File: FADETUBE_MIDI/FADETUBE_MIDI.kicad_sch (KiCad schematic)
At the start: 7 parts, among them J1 B8B-XH-A, J2 B8B-XH-A, J3 B8B-PH-K-S, J4 B8B-PH-K-S, U1 Sparkfun_Pro_Micro

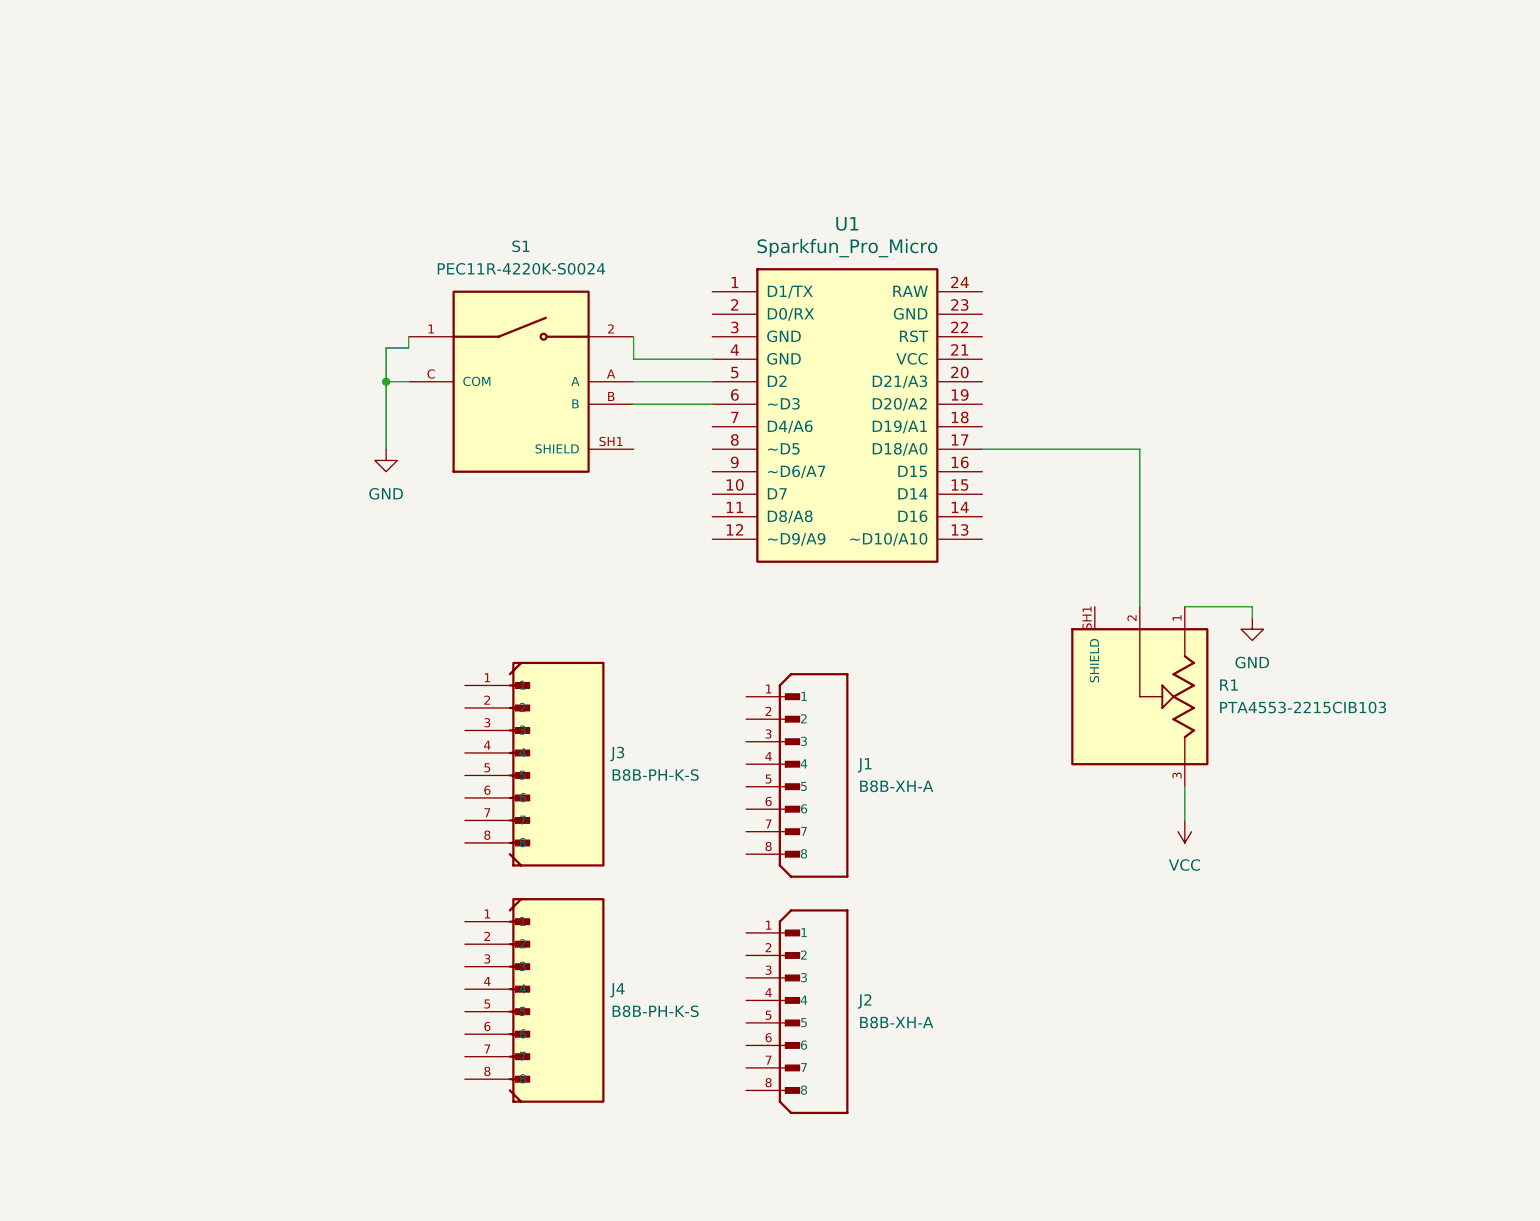
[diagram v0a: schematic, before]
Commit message: updates
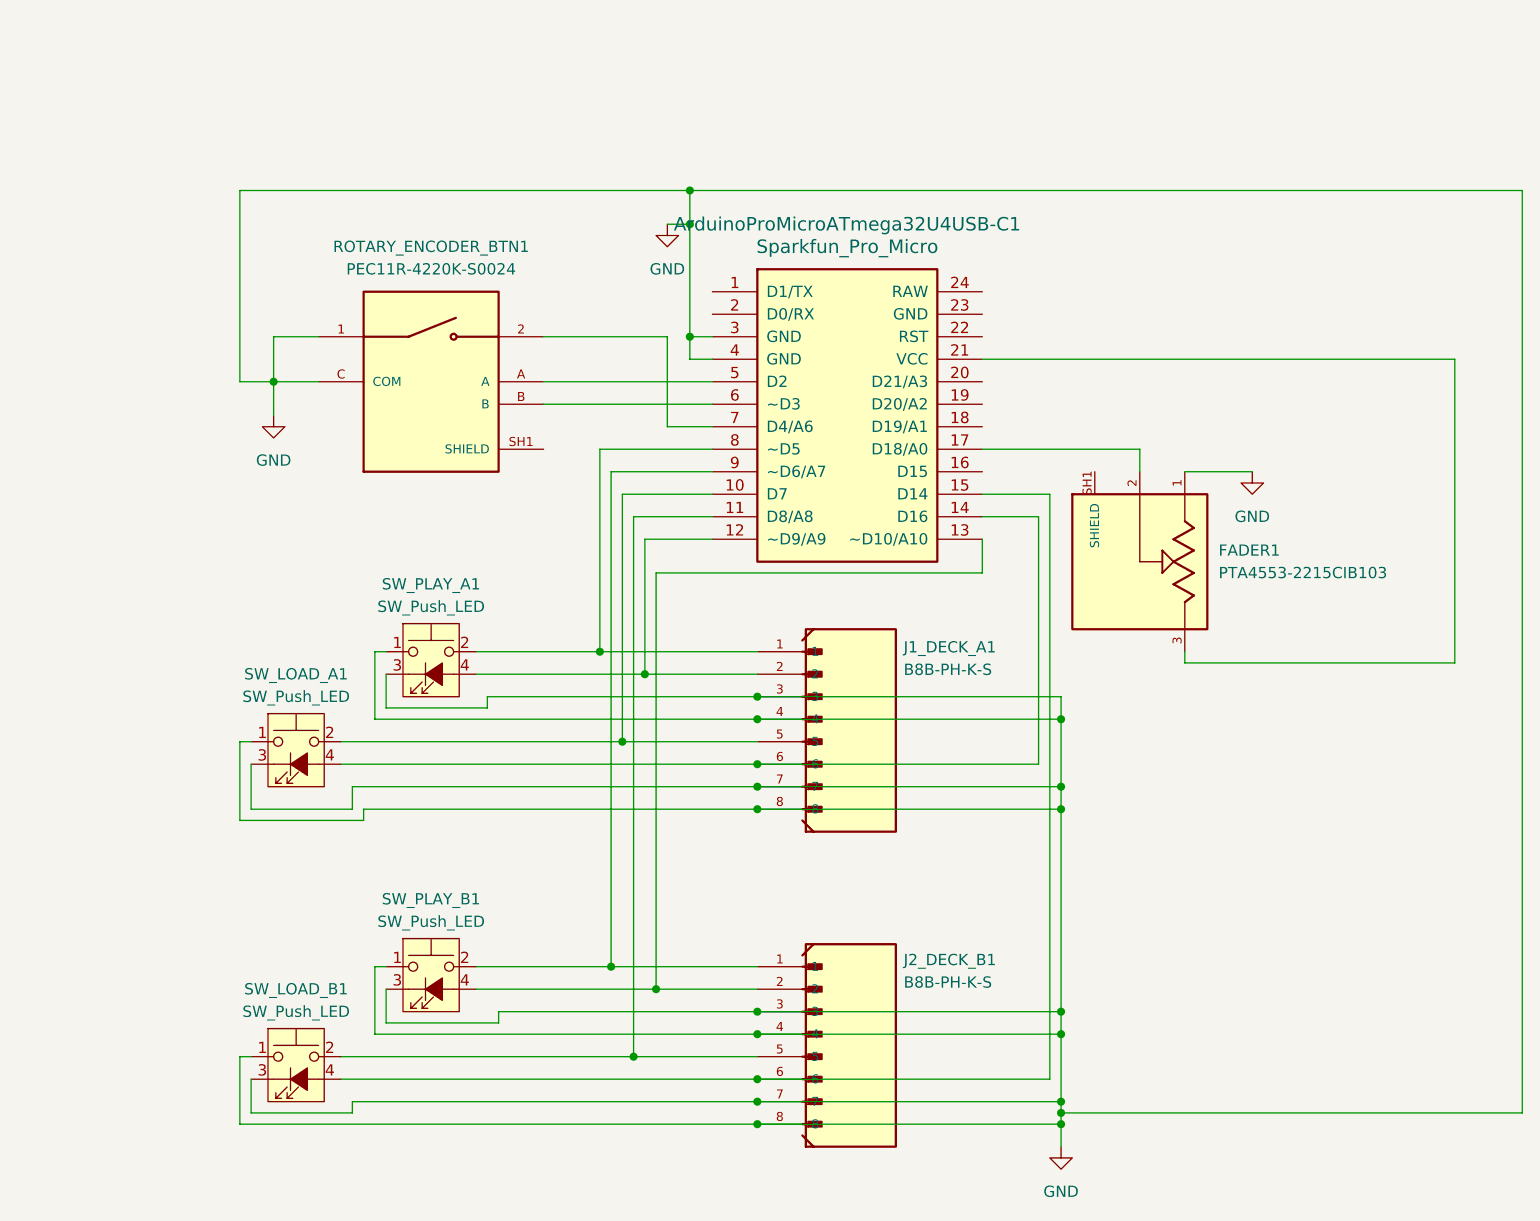
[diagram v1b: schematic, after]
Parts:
- removed J1, J2: B8B-XH-A, FADETUBE_LIBRARY:JST_B8B-XH-A, symbol FADETUBE_LIBRARY:B8B-XH-A
- added SW_LOAD_A1, SW_LOAD_B1, SW_PLAY_A1, SW_PLAY_B1: SW_Push_LED, symbol Switch:SW_Push_LED
- renumbered U1 to ArduinoProMicroATmega32U4USB-C1, R1 to FADER1, J3 to J1_DECK_A1, J4 to J2_DECK_B1, S1 to ROTARY_ENCODER_BTN1
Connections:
- net VCC is gone; now on an unnamed net: FADER1.3
- net GND: now also ArduinoProMicroATmega32U4USB-C1.3 (GND), ArduinoProMicroATmega32U4USB-C1.4 (GND), J1_DECK_A1.3, J1_DECK_A1.4, J1_DECK_A1.7, J1_DECK_A1.8, J2_DECK_B1.3, J2_DECK_B1.4, J2_DECK_B1.7, J2_DECK_B1.8, SW_LOAD_A1.1, SW_LOAD_A1.3 (K), SW_LOAD_B1.1, SW_LOAD_B1.3 (K), SW_PLAY_A1.1, SW_PLAY_A1.3 (K), SW_PLAY_B1.1, SW_PLAY_B1.3 (K)
- net at J1_DECK_A1.1: now also ArduinoProMicroATmega32U4USB-C1.8 (~D5), SW_PLAY_A1.2
- net at J1_DECK_A1.2: now also ArduinoProMicroATmega32U4USB-C1.12 (~D9/A9), SW_PLAY_A1.4 (A)
- net at J1_DECK_A1.5: now also ArduinoProMicroATmega32U4USB-C1.10 (D7), SW_LOAD_A1.2
- net at J1_DECK_A1.6: now also ArduinoProMicroATmega32U4USB-C1.14 (D16), SW_LOAD_A1.4 (A)
- net at J2_DECK_B1.1: now also ArduinoProMicroATmega32U4USB-C1.9 (~D6/A7), SW_PLAY_B1.2
- net at J2_DECK_B1.2: now also ArduinoProMicroATmega32U4USB-C1.13 (~D10/A10), SW_PLAY_B1.4 (A)
- net at J2_DECK_B1.5: now also ArduinoProMicroATmega32U4USB-C1.11 (D8/A8), SW_LOAD_B1.2
- net at J2_DECK_B1.6: now also ArduinoProMicroATmega32U4USB-C1.15 (D14), SW_LOAD_B1.4 (A)
- net at ROTARY_ENCODER_BTN1.2: now also ArduinoProMicroATmega32U4USB-C1.7 (D4/A6); no longer ArduinoProMicroATmega32U4USB-C1.4 (GND)
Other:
- moved on the sheet: FADER1, J1_DECK_A1, J2_DECK_B1, ROTARY_ENCODER_BTN1

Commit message: test smd
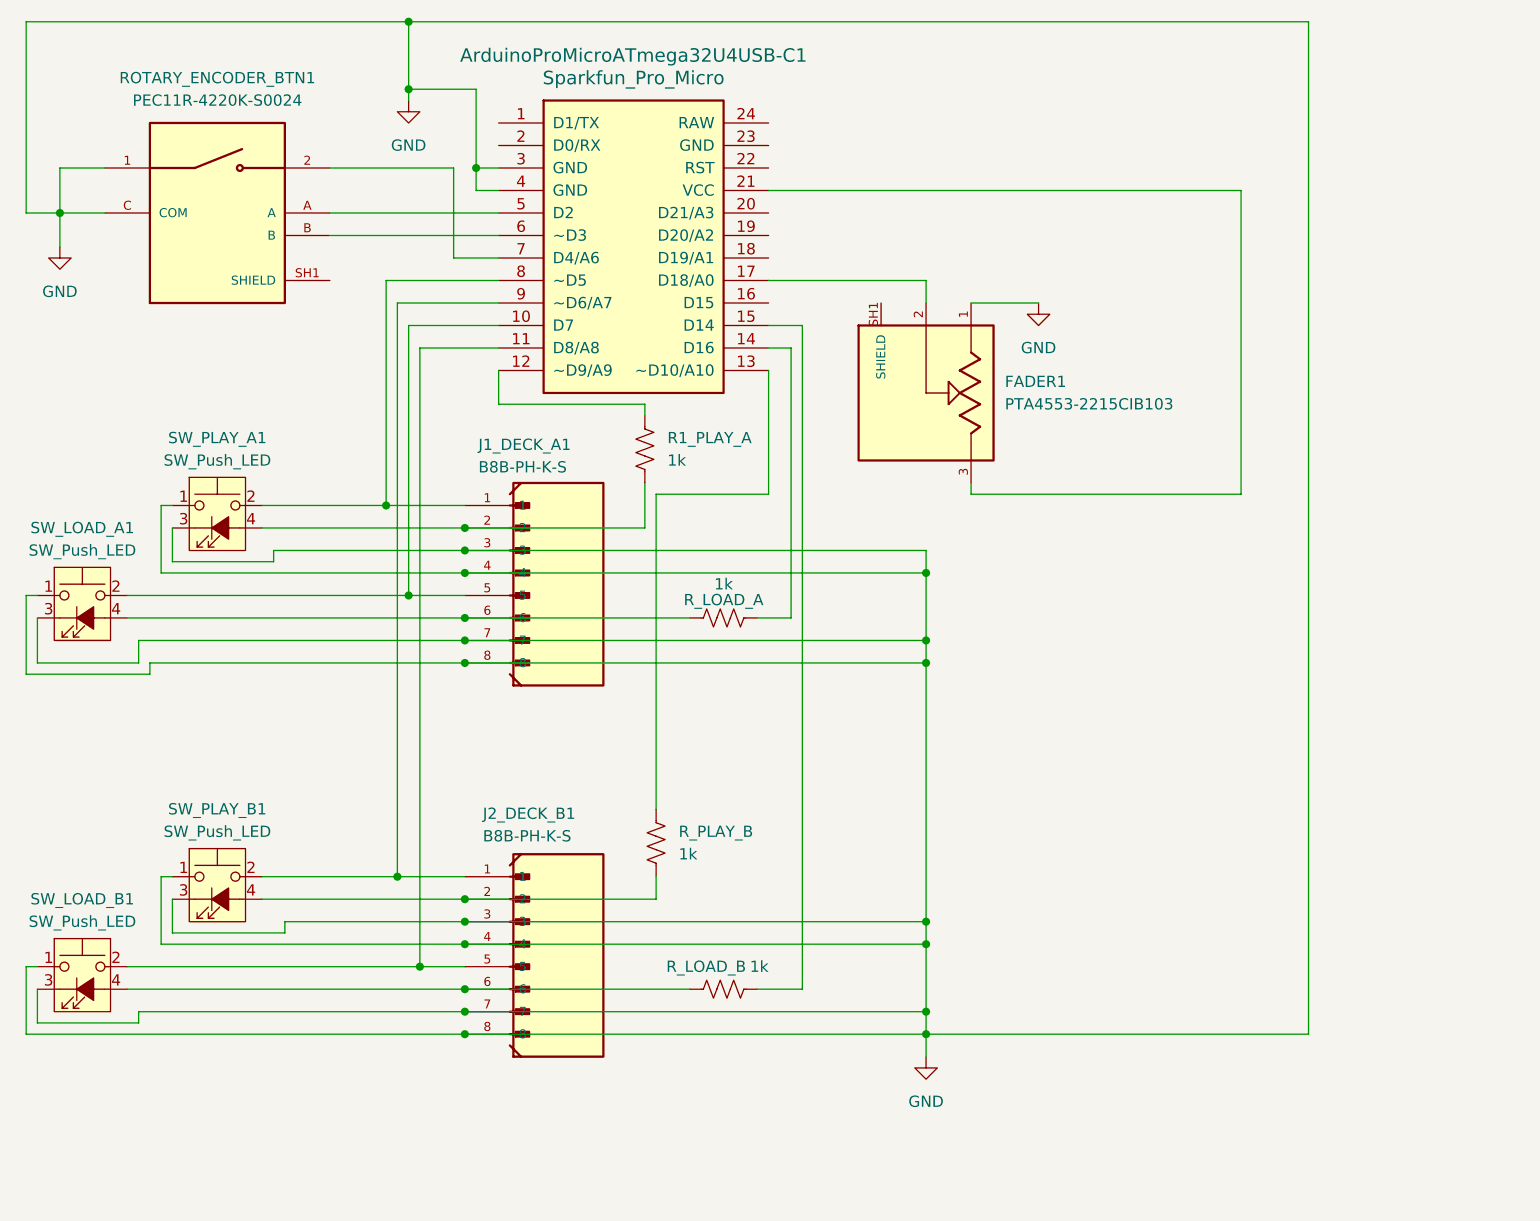
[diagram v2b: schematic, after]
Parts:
- added R1_PLAY_A, R_LOAD_A, R_LOAD_B, R_PLAY_B: 1k, Resistor_SMD:R_0603_1608Metric, symbol Device:R_US
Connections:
- net at J2_DECK_B1.6, SW_LOAD_B1.4 (A): now also R_LOAD_B.1; no longer ArduinoProMicroATmega32U4USB-C1.15 (D14)
- net at J1_DECK_A1.2, SW_PLAY_A1.4 (A): now also R1_PLAY_A.2; no longer ArduinoProMicroATmega32U4USB-C1.12 (~D9/A9)
- net at J1_DECK_A1.6, SW_LOAD_A1.4 (A): now also R_LOAD_A.1; no longer ArduinoProMicroATmega32U4USB-C1.14 (D16)
- net at J2_DECK_B1.2, SW_PLAY_B1.4 (A): now also R_PLAY_B.2; no longer ArduinoProMicroATmega32U4USB-C1.13 (~D10/A10)
- new net: ArduinoProMicroATmega32U4USB-C1.13 (~D10/A10), R_PLAY_B.1
- new net: ArduinoProMicroATmega32U4USB-C1.15 (D14), R_LOAD_B.2
- new net: ArduinoProMicroATmega32U4USB-C1.14 (D16), R_LOAD_A.2
- new net: ArduinoProMicroATmega32U4USB-C1.12 (~D9/A9), R1_PLAY_A.1
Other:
- moved on the sheet: ArduinoProMicroATmega32U4USB-C1, FADER1, J1_DECK_A1, J2_DECK_B1, ROTARY_ENCODER_BTN1, SW_LOAD_A1, SW_LOAD_B1, SW_PLAY_A1, SW_PLAY_B1
